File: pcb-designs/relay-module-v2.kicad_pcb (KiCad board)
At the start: 2 copper layers, 84 x 79.5 mm, 10 parts

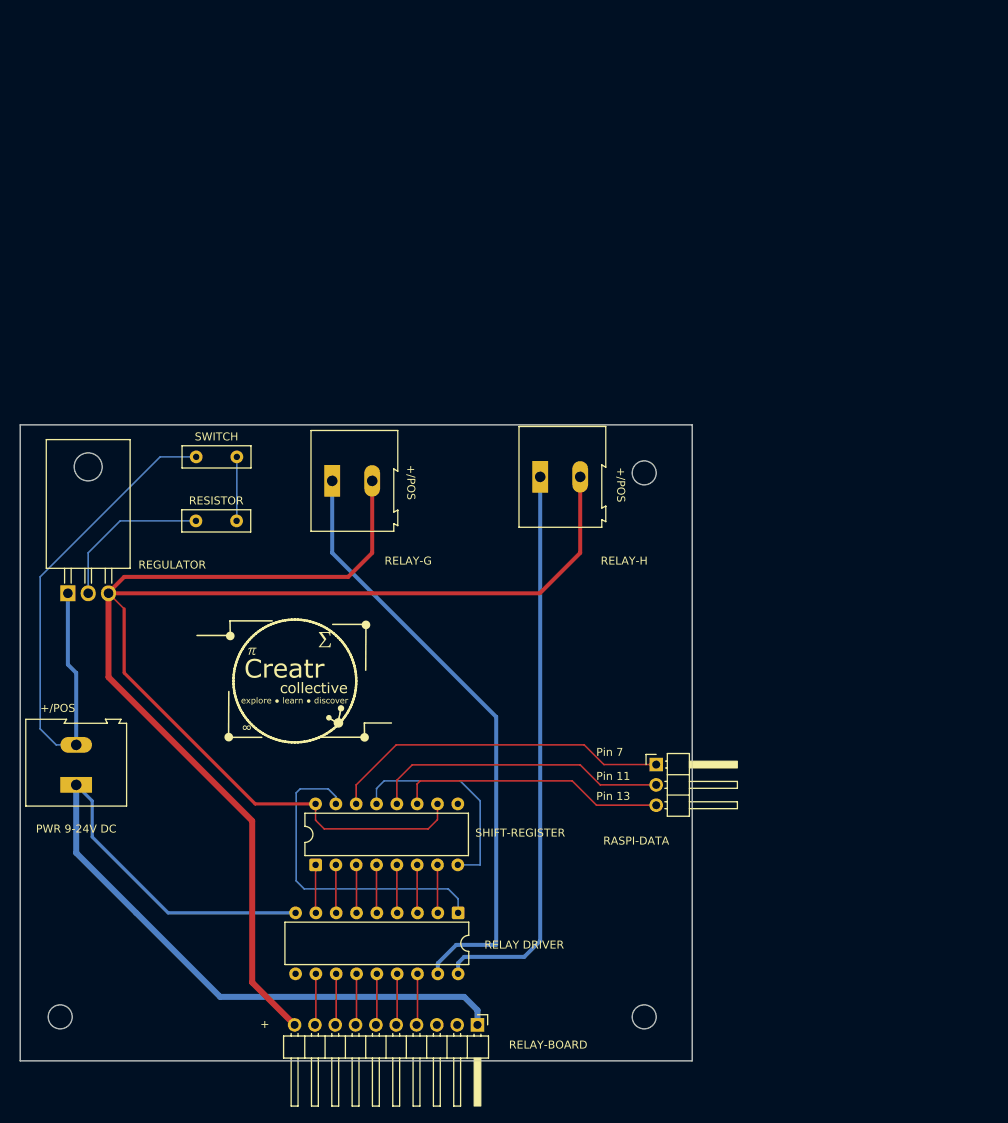
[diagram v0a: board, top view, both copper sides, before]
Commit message: update v2 pcb design
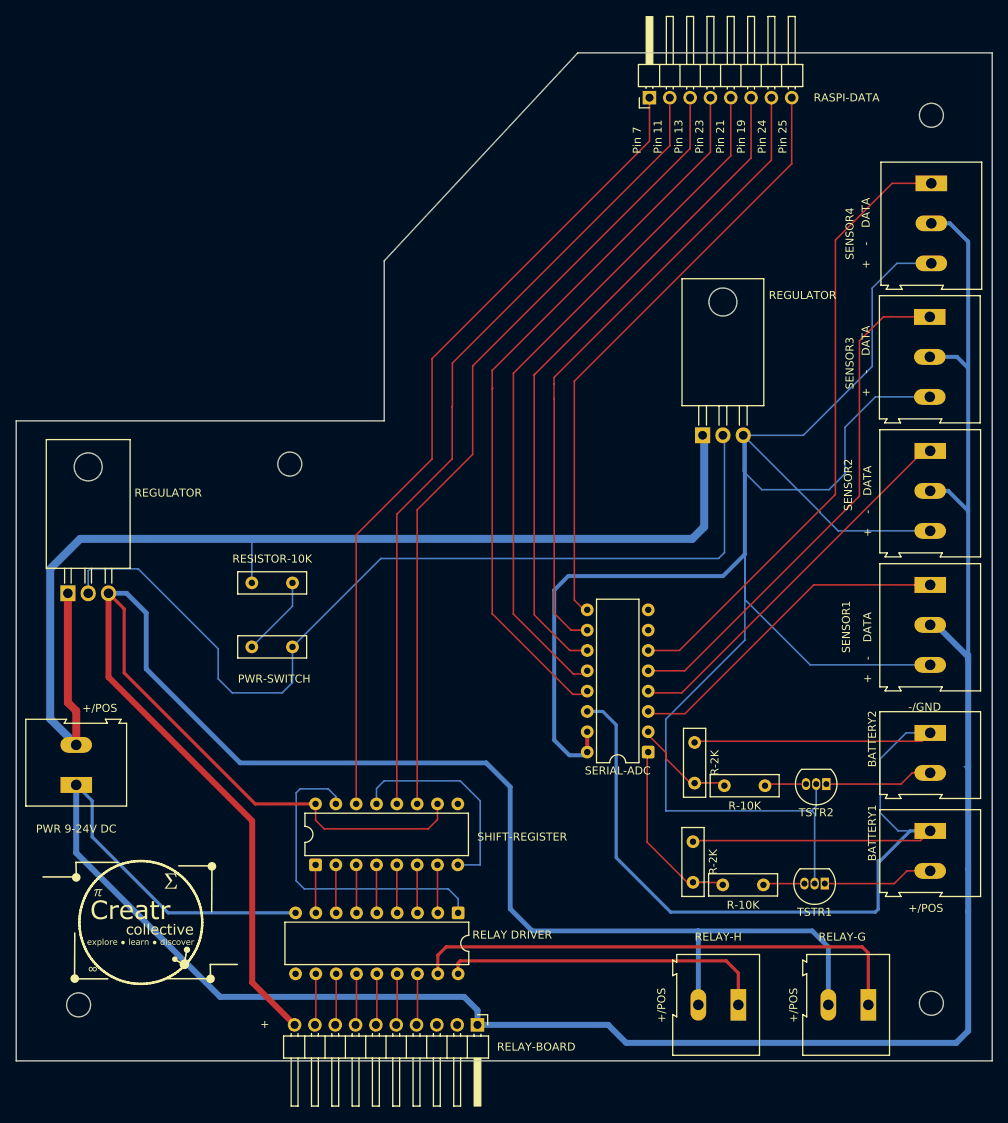
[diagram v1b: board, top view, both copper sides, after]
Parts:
- removed the RASPI-DATA at (134.0, 113.0)
- added BATTERY1: TerminalBlock_Altech_AK300-2_P5.00mm, TerminalBlock:TerminalBlock_Altech_AK300-2_P5.00mm, F.Cu at (168.2, 121.2)
- added BATTERY2: TerminalBlock_Altech_AK300-2_P5.00mm, TerminalBlock:TerminalBlock_Altech_AK300-2_P5.00mm, F.Cu at (168.2, 109.0)
- added R-10K: R_Box_L8.4mm_W2.5mm_P5.08mm, Resistor_THT:R_Box_L8.4mm_W2.5mm_P5.08mm, F.Cu at (147.6, 115.6)
- added R-10K: R_Box_L8.4mm_W2.5mm_P5.08mm, Resistor_THT:R_Box_L8.4mm_W2.5mm_P5.08mm, F.Cu at (147.4, 128.0)
- added R-2K: R_Box_L8.4mm_W2.5mm_P5.08mm, Resistor_THT:R_Box_L8.4mm_W2.5mm_P5.08mm, F.Cu at (138.8, 110.2)
- added R-2K: R_Box_L8.4mm_W2.5mm_P5.08mm, Resistor_THT:R_Box_L8.4mm_W2.5mm_P5.08mm, F.Cu at (138.6, 122.6)
- added RASPI-DATA: PinHeader_1x08_P2.54mm_Horizontal, Connector_PinHeader_2.54mm:PinHeader_1x08_P2.54mm_Horizontal, F.Cu at (133.2, 29.6)
- added REF**: TerminalBlock_Altech_AK300-3_P5.00mm, TerminalBlock:TerminalBlock_Altech_AK300-3_P5.00mm, F.Cu at (168.4, 40.3)
- added REGULATOR: TO-220-3_Horizontal_TabDown, Package_TO_SOT_THT:TO-220-3_Horizontal_TabDown, F.Cu at (139.8, 71.8)
- added SENSOR1: TerminalBlock_Altech_AK300-3_P5.00mm, TerminalBlock:TerminalBlock_Altech_AK300-3_P5.00mm, F.Cu at (168.2, 90.5)
- added SENSOR2: TerminalBlock_Altech_AK300-3_P5.00mm, TerminalBlock:TerminalBlock_Altech_AK300-3_P5.00mm, F.Cu at (168.2, 73.8)
- added SENSOR3: TerminalBlock_Altech_AK300-3_P5.00mm, TerminalBlock:TerminalBlock_Altech_AK300-3_P5.00mm, F.Cu at (168.2, 57.0)
- added SERIAL-ADC: CERDIP-16_W7.62mm_SideBrazed, Package_DIP:CERDIP-16_W7.62mm_SideBrazed, F.Cu at (133.0, 111.4)
- added TSTR1: TO-92_Inline, Package_TO_SOT_THT:TO-92_Inline, F.Cu at (155.1, 127.8)
- added TSTR2: TO-92_Inline, Package_TO_SOT_THT:TO-92_Inline, F.Cu at (155.3, 115.4)
- moved RELAY-G 93.7 mm to (160.5, 143.0), turned to 180 degrees
- moved RELAY-H 70.5 mm to (144.3, 143.0), turned to 180 degrees
- moved PWR-SWITCH 26.6 mm to (88.5, 98.2), turned to 180 degrees
- moved RESISTOR-10K 14.3 mm to (88.5, 90.2), turned to 180 degrees
- renumbered SWITCH to PWR-SWITCH, RESISTOR to RESISTOR-10K
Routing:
- net (no net): track 853.5 -> 2570.2 mm
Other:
- board size 84 x 79.5 mm -> 122 x 126 mm
- board text added: "+ - DATA"
- board text added: "-/GND"
- board text added: "Pin 19"
- board text added: "Pin 21"
- board text added: "Pin 23"
- board text added: "Pin 24"
- board text added: "Pin 25"
- board text added: "SENSOR3"
- board text added: "SENSOR4"
